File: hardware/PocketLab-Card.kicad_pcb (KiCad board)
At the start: 4 copper layers, 85.6 x 54 mm, 266 parts, among them J1 USB-C DATA/POWER, J2 microSD, J3 EXTERNAL 400uH LF COIL, J4 PROTECTED 1S LiPo 3.7V, J5 30-PIN 2.54mm DUPONT GRID, J8 ER-OLED0.42-1W 72x40 SSD1306B, Q1 AO3400A IR DRIVER, Q2 CSD16406Q3 DISCHARGE, Q3 CSD16406Q3 CHARGE, SW1 RESET, SW2 BOOT, SW3 UP, SW4 DOWN, SW5 MAIN POWER OFF / ON, SW6 PAIR, SW7 SELECT, U1 ESP32-S3-WROOM-1-N8R2, U10 BMI270 (FULL OPTION), U11 BMP390 (FULL OPTION), U12 PCF8563T, U13 TSOP75338WTR 38kHz, U14 BQ29700DSE, U15 TPS2553DBVR 500mA LIMIT, U16 USBLC6-4SC6Y, U17 TPS22919DCKR LF 5V LOAD SWITCH, U18 TCA9534PWR INTERNAL CONTROL, U19 SRV05-4MR6T1G SD ESD, U2 PN5321A3HN/C106, U20 SN74AHCT1G126DBVR RGB LEVEL S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, U21 SN74AHCT125PWR LF 3V3-TO-5V, U22 SN74LVC1G17DBVR LF 5V-TO-3V3, U23 ATECC608C-SSHDA-T, U24 SRV05-4MR6T1G J5 BUS ESD, U25 SRV05-4MR6T1G J5 SPI ESD, U3 E07-900MM10S 855-925MHz, U4 HTRC11001T/03EE,11 125kHz, U5 BQ24074RGTR, U6 TPS63070RNMR 3V3, U7 TPS61023DRLR 5V BOOST, U8 MAX17048G+T10, U9 TCA9535PWR, Y301 27.12MHz crystal (pins 2/4 sh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, Y501 4MHz 5V CMOS OSCILLATOR, Y701 32.768kHz CL=7pF

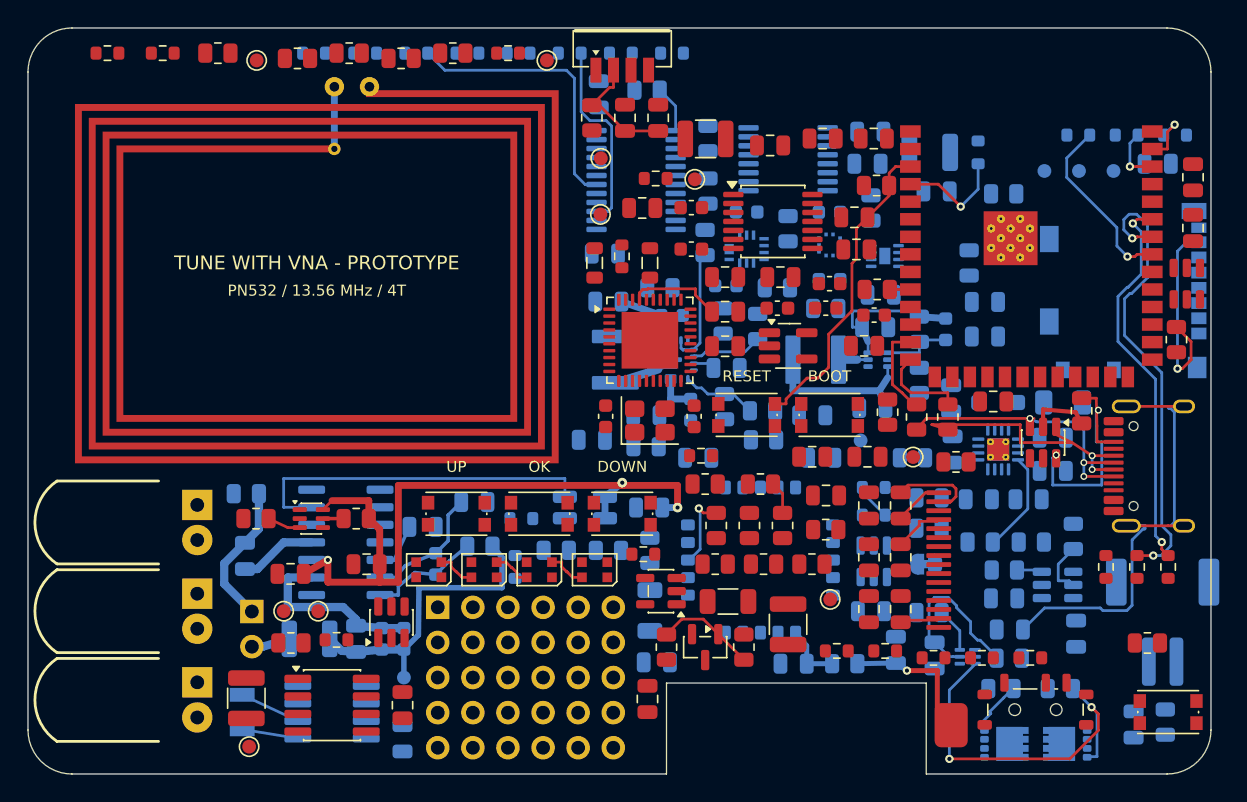
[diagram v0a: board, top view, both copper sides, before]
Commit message: Save shared-SPI LF and plane-fanout checkpoint
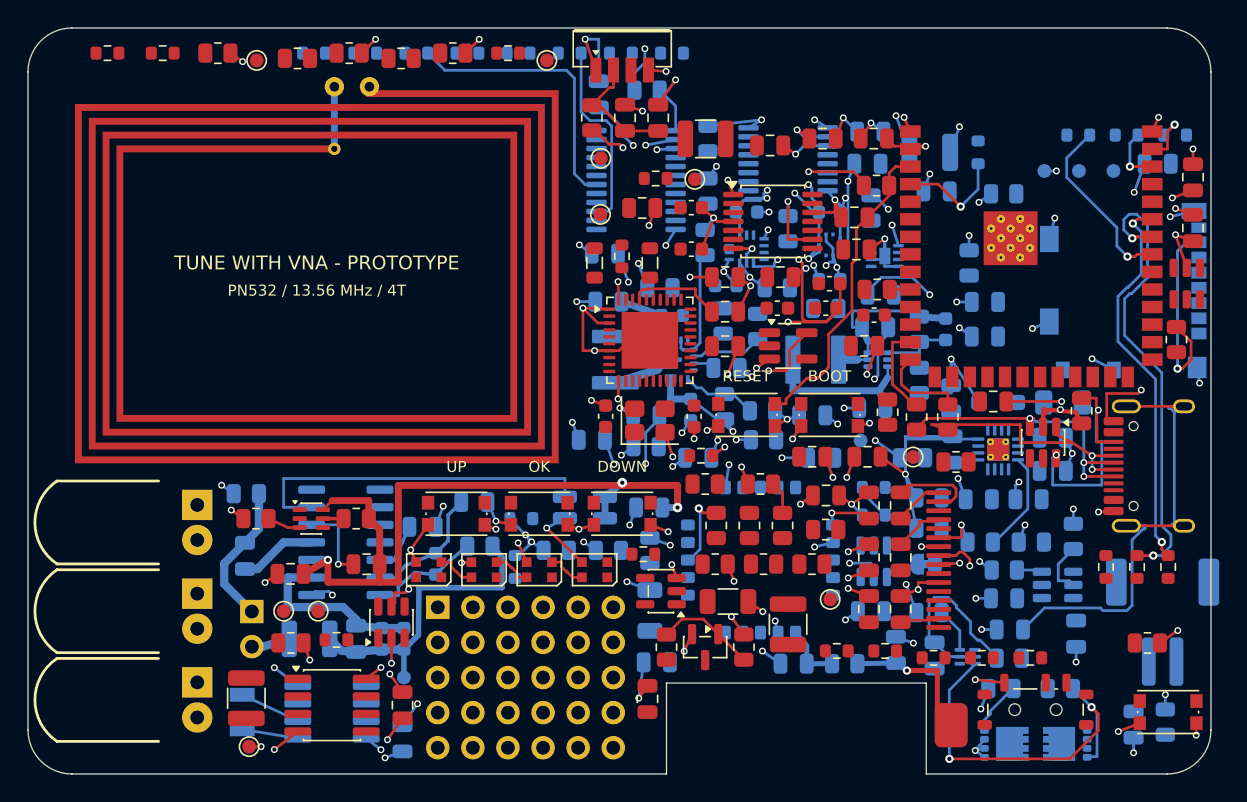
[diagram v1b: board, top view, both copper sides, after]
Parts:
- C515: value 100nF AHCT supply -> 100nF LV-AT supply
- U21: value SN74AHCT125PWR LF 3V3-TO-5V -> SN74LV125ATPWR LF/SPI 3V3-TO-5V IOFF
- U22: value SN74LVC1G17DBVR LF 5V-TO-3V3 -> SN74LVC1G126DBVR LF 5V-TO-3V3 TRI-STATE
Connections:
- U1 pad 11: /LF_SCLK_3V3 -> unconnected-(U1-IO18-Pad11)
- U1 pad 23: /LF_DOUT_3V3 -> unconnected-(U1-IO21-Pad23)
- U1 pad 28: /LF_DIN_3V3 -> unconnected-(U1-IO35-Pad28)
- U21 pad 2: /LF_SCLK_3V3 -> /SPI_MOSI
- U21 pad 3: /LF_SCLK_5V -> /LF_DIN_5V
- U21 pad 5: /LF_DIN_3V3 -> /SPI_SCK
- U21 pad 6: /LF_DIN_5V -> /LF_SCLK_5V
- U22 pad 1: unconnected-(U22-NC-Pad1) -> /LF_RFID_EN
- U22 pad 4: /LF_DOUT_3V3 -> /SPI_MISO
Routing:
- net /GND: track 4.54 -> 328.8 mm, vias 0 -> 136
- net /+3V3: track 2.90 -> 127.9 mm, vias 0 -> 55
